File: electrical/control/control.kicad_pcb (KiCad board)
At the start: 2 copper layers, 33 x 48 mm, 42 parts, among them J1 USB4105-GF-A, J2 SWD, J3 TC2030-NL, J4 UART, J5 QWIIC, SW1 228EMSARGFR, U1 USBLC6-2P6, U2 LP5912-3.3DRV, U3 W25Q16JVUXIQ, U4 RP2040, U5 ABPMRRV060MG2A3, Y1 ABM8-272-T3

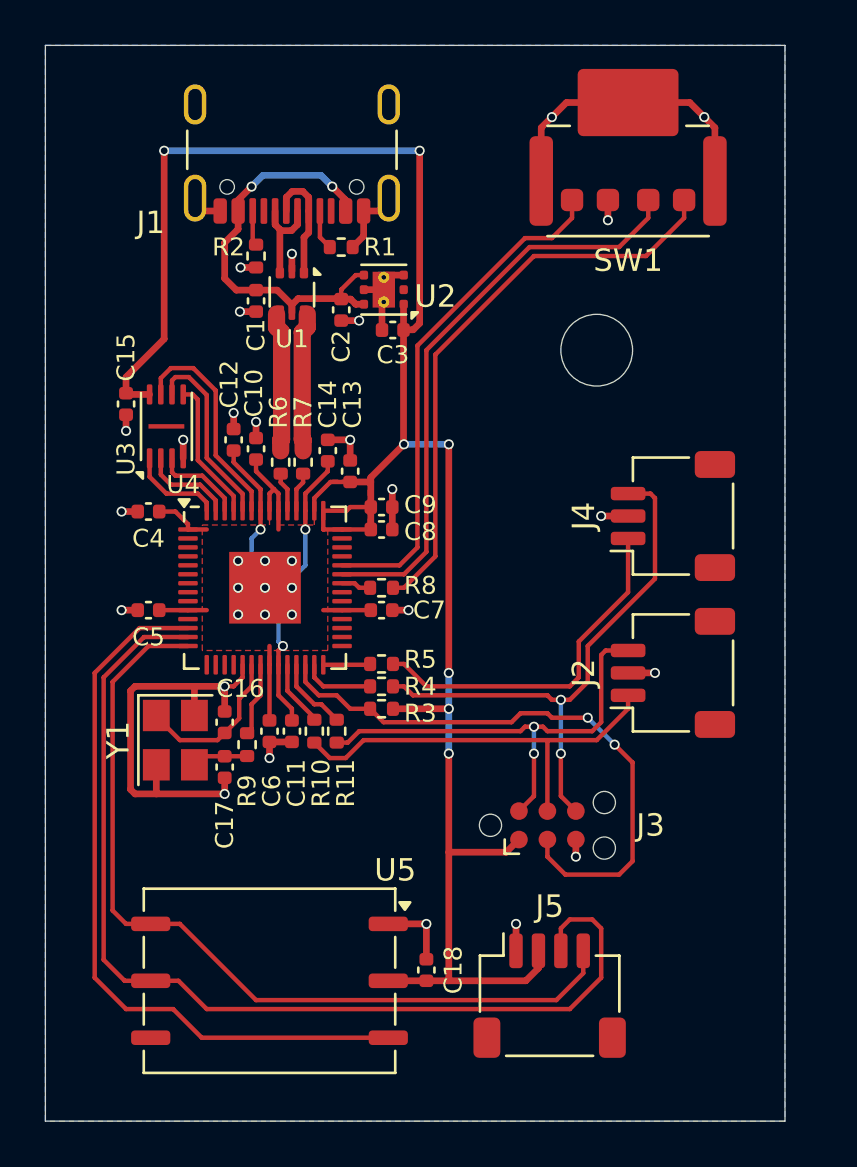
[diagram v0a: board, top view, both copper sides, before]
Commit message: More PCB tweaks
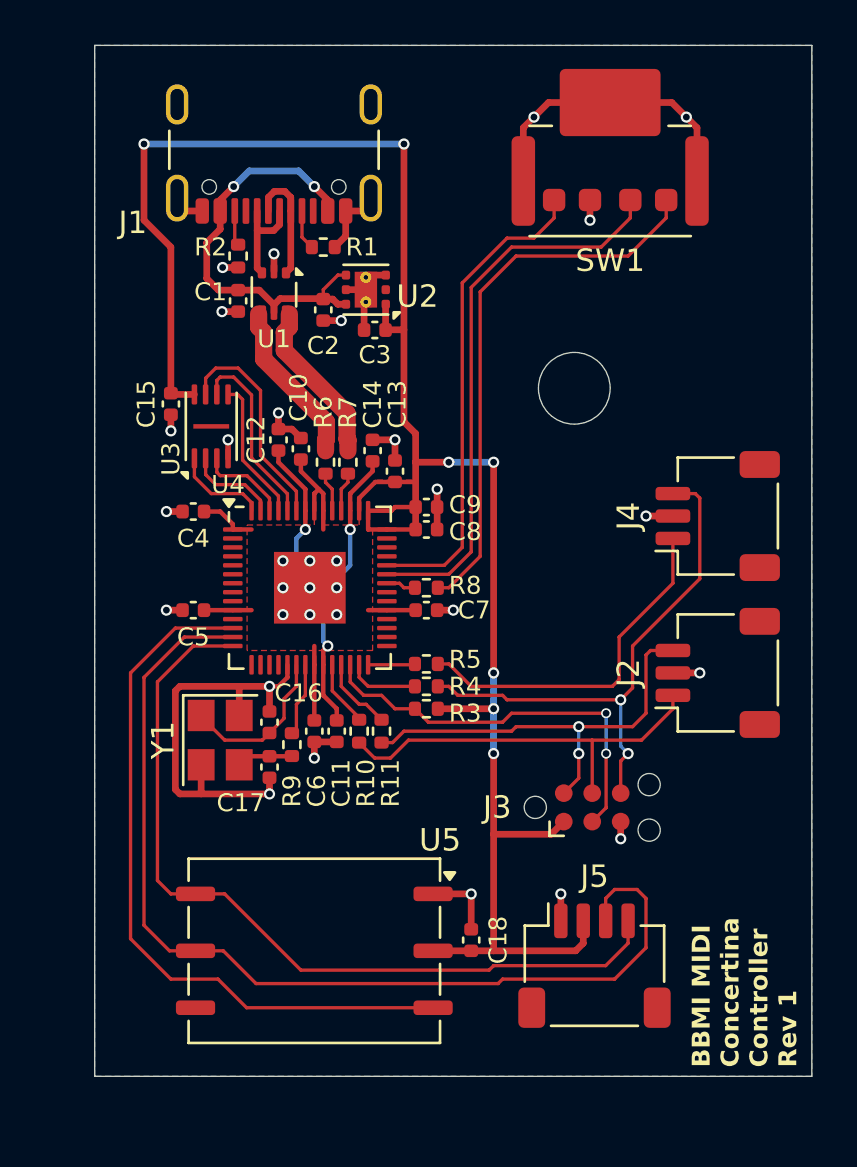
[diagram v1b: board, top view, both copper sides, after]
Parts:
- moved J5 2.41 mm to (166.5, 109.1)
- moved C18 2.41 mm to (161.0, 107.9)
- moved U5 2.41 mm to (154.0, 108.4)
- moved J3 2.15 mm to (166.4, 102.0)
- moved C10 2.00 mm to (153.4, 86.0)
- moved C11 2.00 mm to (155.0, 98.6)
- moved C12 2.00 mm to (152.4, 85.6)
- moved C13 2.00 mm to (157.6, 87.0)
- moved C14 2.00 mm to (156.6, 86.1)
- moved C15 2.00 mm to (147.6, 84.0)
- moved C16 2.00 mm to (152.0, 98.2)
- moved C17 2.00 mm to (152.0, 100.2)
- moved C4 2.00 mm to (148.6, 88.8)
- moved C5 2.00 mm to (148.6, 93.2)
- moved C6 2.00 mm to (154.0, 98.6)
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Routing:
- net RUN: track 26.7 -> 18.2 mm
- net I2C_SCL: track 38.4 -> 37.0 mm
- net SWDIO: track 20.7 -> 19.5 mm
- net Net-(U4-GPIO25): track 26.3 -> 25.2 mm
- net Net-(R8-Pad2): track 25.9 -> 24.7 mm
- net USB_D-: track 6.22 -> 7.37 mm
- net Net-(U4-GPIO26_ADC0): track 22.8 -> 21.6 mm
- net USB_D+: track 6.22 -> 7.37 mm
- net I2C_SDA: track 46.1 -> 45.2 mm
- net SWCLK: track 19.0 -> 18.2 mm
- net PRESSURE_INT: track 32.8 -> 32.0 mm
- net UART_TX: track 25.2 -> 24.6 mm
- net GND: track 62.5 -> 63.0 mm, vias 33 -> 32
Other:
- board size 33 x 48 mm -> 32 x 46 mm
- board text added: "BBMI MIDI Concertina Controller Rev 1"
